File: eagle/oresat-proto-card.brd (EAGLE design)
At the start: 99.8 x 94.7 mm, 120 parts, among them J1 J-SAMTEC-TFM-110-X1-XXX-D-RA, J2 U.FL, J3 U.FL, J4 U.FL, J5 DNP, J6 J-SAMTEC-TFM-120-X1-XXX-D-RA, J7 FTSH-105-XX-X-DV-K, Q1 DMP2240UDM, Q3 MOSFET-PCH-SOT23-6, Q4 MOSFET-PCH-SOT23-6, Q5 PMV45EN, Q6 PMV45EN, U2 TCAN330, U3 MAX7310ATE, U4 MAX4211FETE, U5 TPS62111RSA, U6 STM32F042K6, U8 MIC842LYC5, U9 MIC842LYC5, X1 16MHZ-2.5x2mm

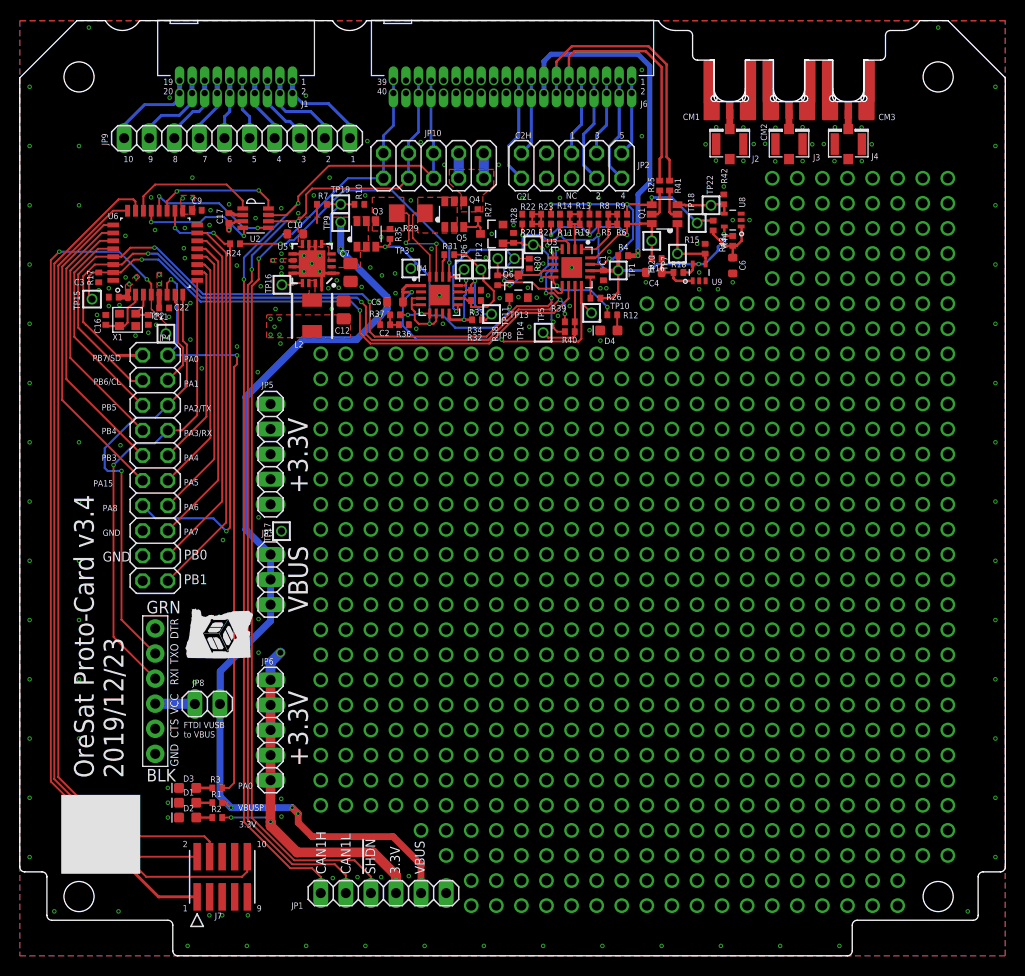
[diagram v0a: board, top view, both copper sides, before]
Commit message: protocard preliminary rev 3.5
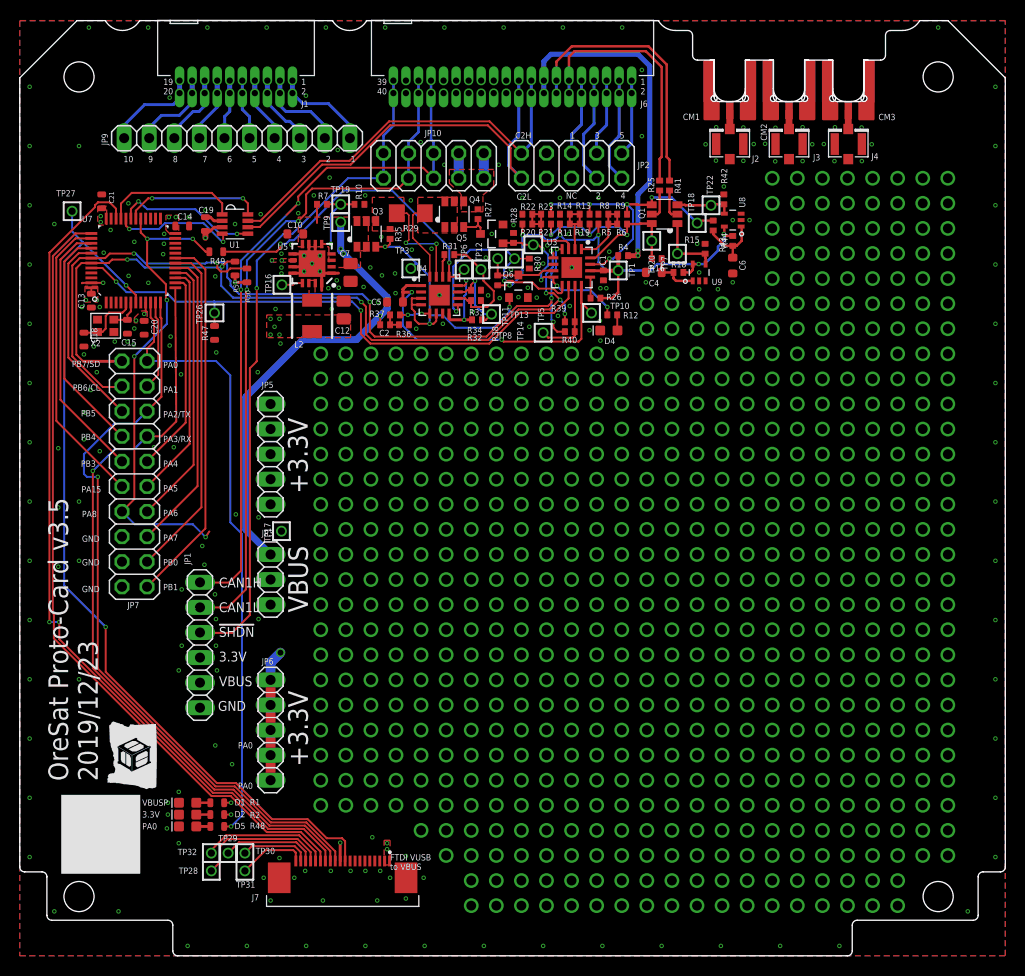
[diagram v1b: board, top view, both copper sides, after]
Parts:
- removed C11, C16: 20p, rcl_custom:.0402-B-NOSILK
- removed C17, C22, C3, C9: 100n, rcl_custom:.0402-B-NOSILK
- removed D3: AMBER, SparkFun-LED:LED-0603
- removed J5: DNP, SparkFun-Connectors:6_PIN_SERIAL_TARGET_SIDE_W_SILK
- removed JP4: (no value), pinhead:2X10
- removed JP8: (no value), pinhead:1X02
- removed R17: 10k, rcl_custom:.0402-B-NOSILK
- removed R24: 10k, rcl:R0402
- removed R3: 2.7k, rcl_custom:.0402-B-NOSILK
- removed TP15, TP2: TEST-POINT, Tova:2MM-TEST-POINT
- removed U2: TCAN330, TCAN330:SOT23-8_TI-DCN
- removed U6: STM32F042K6, STM32F042K:QFP32-7X7
- removed X1: 16MHZ-2.5x2mm, low-gain-radio:CRYSTAL_2.5X2
- added C13, C14, C19, C20, C21: 100n, oresat-rcl:.0603-C-NOSILK
- added C15, C18: 20p, oresat-rcl:.0603-C-NOSILK
- added D5: AMBER, SparkFun-LED:LED-0603
- added JP7: (no value), pinhead:2X10
- added R47, R49: 10k, oresat-rcl:.0603-C-NOSILK
- added R48, R50, R51: 2.7k, oresat-rcl:.0603-C-NOSILK
- added TP26, TP27, TP28, TP29, TP30, TP31, TP32: TEST-POINT, Tova:2MM-TEST-POINT
- added U1: TCAN330, TCAN330:SOT23-8_TI-DCN
- added U7: STM32F091C, U-ST-STM32F091C-uC:STM32F091C
- added X2: 16MHZ-2.5x2mm, low-gain-radio:CRYSTAL_2.5X2
- J7: value FTSH-105-XX-X-DV-K -> ORESAT-DEBUG-CONNECTOR-CARD; device J-Samtec-FTSH-105-XXX-DV-K-ARM-SWD:CON10_2X5_DUK_FTSH -> oresat-edge_connector:TE_2-1734592-0
- R1, R2: device rcl_custom:.0402-B-NOSILK -> oresat-rcl:.0603-C-NOSILK
- moved JP1 31.2 mm to (18.2, 31.5), turned to 270 degrees
- moved J7 12.2 mm to (32.7, 7.90), turned to 180 degrees
- moved D2 0.30 mm to (17.0, 14.3)
- moved R2 0.30 mm to (20.0, 14.3)
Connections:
- removed net CRYSTALIN: C16.1, U6.2, X1.1
- removed net CRYSTALOUT: C11.1, U6.3, X1.3
- removed net N$1: D3.A, R3.1
- removed net N$406: J5.P$4, JP8.2
- new net CRYSTALIN1: C18.1, U7.5, X2.1
- new net CRYSTALOUT1: C15.1, U7.6, X2.3
- new net N$522: D5.A, R48.1
- new net N$523: J7.20, TP31.1
- new net N$524: J7.19, TP30.1
- new net N$525: J7.18, TP29.1
- new net N$526: J7.17, TP28.1
- new net N$527: J7.16, TP32.1
- new net VBAT: U7.1
- net 3.3V: now also C13.2, C14.2, C19.2, C20.2, C21.2, J7.11, R50.2, R51.2, U1.3, U7.24, U7.36, U7.48, U7.9; no longer C17.2, C22.2, C3.2, C9.2, J7.1, U2.3, U6.1, U6.17, U6.5
- net BOOT0: now also R47.2, TP26.1, U7.44; no longer R17.2, TP15.1, U6.31
- net CAN1_H: no longer U2.7
- net CAN1_L: no longer U2.6
- net CAN2_H: now also U1.7
- net CAN2_L: now also U1.6
- net CAN_RX: now also U1.4, U7.32; no longer U2.4, U6.21
- net CAN_SHDN: now also U1.5, U7.31; no longer U2.5, U6.20
- net CAN_SILENT: now also U1.8, U7.30; no longer U2.8, U6.19
- net CAN_TX: now also U1.1, U7.33; no longer U2.1, U6.22
- net GND: now also C13.1, C14.1, C15.2, C18.2, C19.1, C20.1, C21.1, D5.C, J7.6, J7.PAD1, J7.PAD2, JP7.15, JP7.17, JP7.19, R47.1, U1.2, U7.23, U7.35, U7.47, U7.8, X2.2, X2.4; no longer C11.2, C16.2, C17.1, C22.1, C3.1, C9.1, D3.C, J5.P$6, J7.5, JP4.15, JP4.17, JP4.19, R17.1, U2.2, U6.16, U6.32, X1.2, X1.4
- net NRESET: now also TP27.1, U7.7; no longer TP2.1, U6.4
- net PA0: now also JP7.2, R48.2, U7.10; no longer JP4.2, R3.2, U6.6
- net PA1: now also JP7.4, U7.11; no longer JP4.4, U6.7
- net PA15: now also JP7.11, U7.38; no longer JP4.11, U6.25
- net PA2/USART2_TX: now also J7.12, JP7.6, U7.12; no longer J5.P$2, JP4.6, U6.8
- net PA3/USART2_RX: now also J7.13, JP7.8, U7.13; no longer J5.P$3, JP4.8, U6.9
- net PA4: now also JP7.10, U7.14; no longer JP4.10, U6.10
- net PA5/SPI1_SCK: now also JP7.12, U7.15; no longer JP4.12, U6.11
- net PA6/SPI1_MISO: now also JP7.14, U7.16; no longer JP4.14, U6.12
- net PA7/SPI1_MOSI: now also JP7.16, U7.17; no longer JP4.16, U6.13
- net PB0: now also JP7.18, U7.18; no longer JP4.18, U6.14
- net PB1: now also JP7.20, U7.19; no longer JP4.20, U6.15
- net PB3: now also JP7.9, U7.39; no longer JP4.9, U6.26
- net PB4: now also JP7.7, U7.40; no longer JP4.7, U6.27
- net PB5: now also JP7.5, U7.41; no longer JP4.5, U6.28
- net PB6/SCL: now also JP7.3, R50.1, U7.42; no longer JP4.3, U6.29
- net PB7/SDA: now also JP7.1, R51.1, U7.43; no longer JP4.1, U6.30
- net POUT: now also R49.1; no longer R24.1
- net POUTPROT: now also JP7.13, R49.2, U7.29; no longer JP4.13, R24.2, U6.18
- net SWCLK: now also J7.15, U7.37; no longer J7.4, U6.24
- net SWDIO: now also J7.14, U7.34; no longer J7.2, U6.23
- net VBUS: now also J7.1, J7.2
- net VBUSP: no longer JP8.1
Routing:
- net VBUS: track 5.08 -> 80.6 mm, vias 0 -> 2
- net CAN2_L: track 10.9 -> 46.2 mm
- net CAN1_L: track 104.9 -> 70.0 mm
- net CAN1_H: track 106.4 -> 72.0 mm
- net CAN2_H: track 7.77 -> 41.0 mm
- net PA2/USART2_TX: track 44.1 -> 75.5 mm
- net !SD: track 99.4 -> 68.6 mm
- net 3.3V: track 53.8 -> 23.4 mm, vias 18 -> 20
- net PA3/USART2_RX: track 47.6 -> 76.8 mm
- net VBUSP: track 103.8 -> 81.1 mm, vias 6 -> 4
- net N$526: track 0.00 -> 13.8 mm
- net N$527: track 0.00 -> 13.1 mm
- net N$525: track 0.00 -> 9.65 mm
- net N$524: track 0.00 -> 7.09 mm
- net N$523: track 0.00 -> 6.97 mm
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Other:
- board text added: "OreSat Proto-Card v3.5"
- board text removed: "OreSat Proto-Card v3.4"
